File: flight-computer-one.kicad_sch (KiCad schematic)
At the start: 8 parts, among them J1 LEFT_BANK, J2 RIGHT_BANK

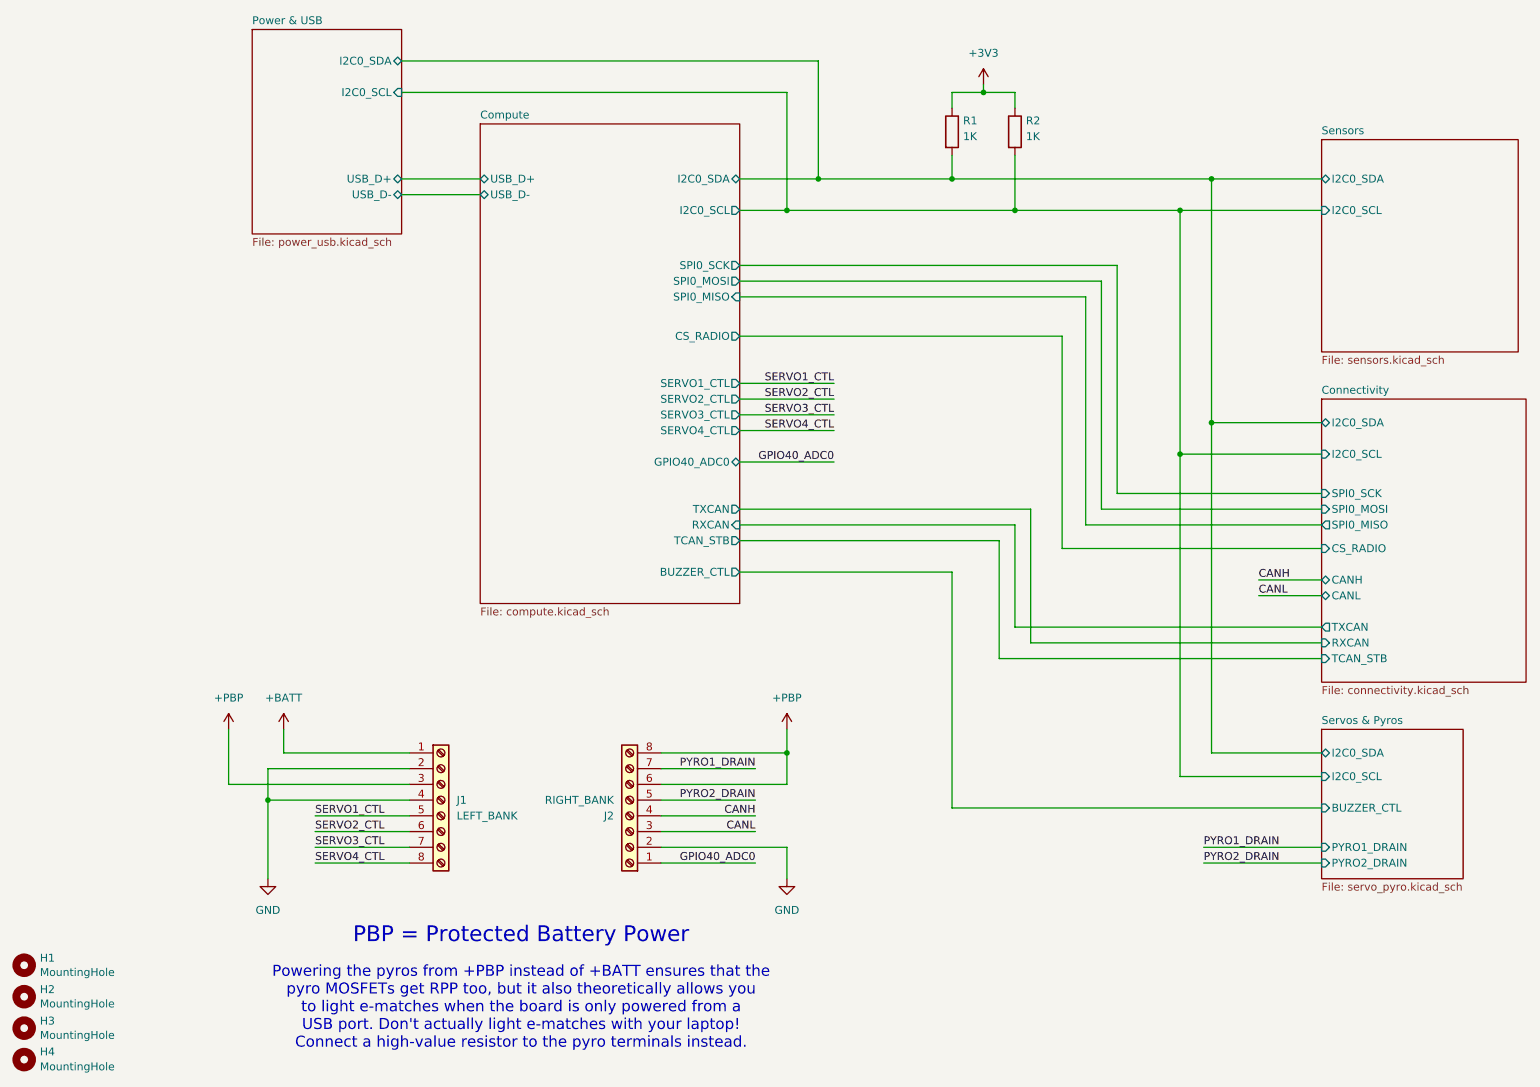
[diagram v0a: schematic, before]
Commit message: Final schematic changes
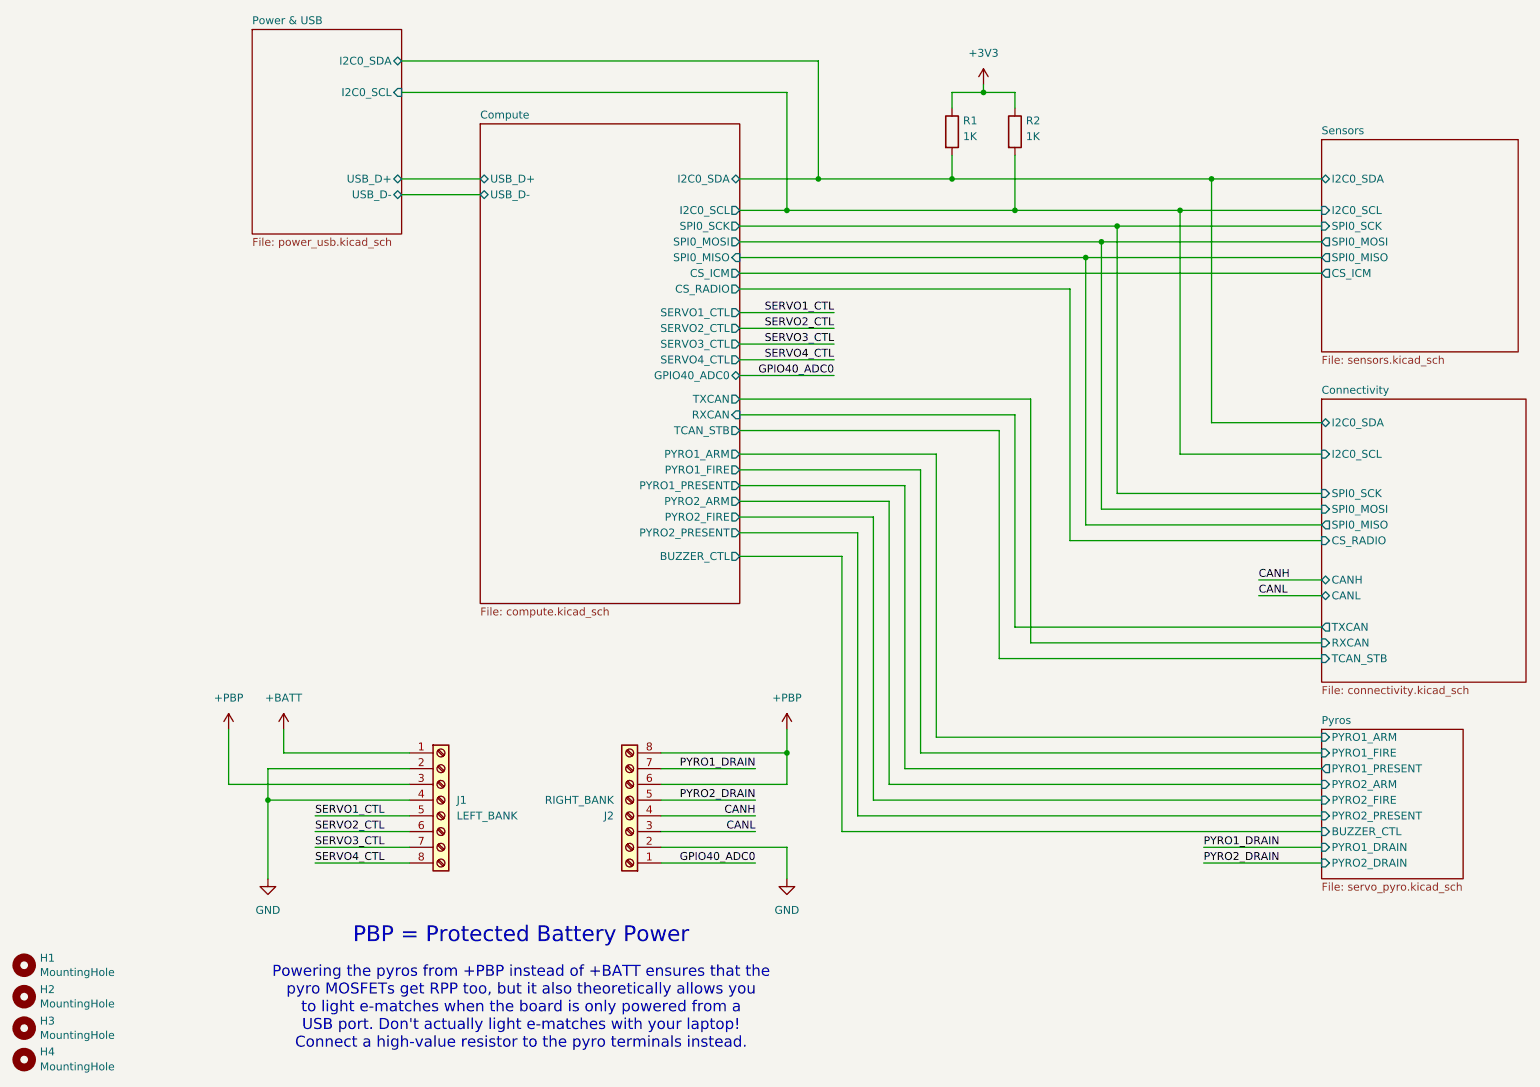
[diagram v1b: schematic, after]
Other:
- sheet Servos & Pyros renamed Pyros
- sheet Compute ports: added CS_ICM, PYRO1_ARM, PYRO1_FIRE, PYRO1_PRESENT, PYRO2_ARM, PYRO2_FIRE, PYRO2_PRESENT; removed none
- sheet Pyros ports: added PYRO1_ARM, PYRO1_FIRE, PYRO1_PRESENT, PYRO2_ARM, PYRO2_FIRE, PYRO2_PRESENT; removed I2C0_SCL, I2C0_SDA
- sheet Sensors ports: added CS_ICM, SPI0_MISO, SPI0_MOSI, SPI0_SCK; removed none
